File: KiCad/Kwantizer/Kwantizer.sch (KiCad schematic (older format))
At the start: 29 parts

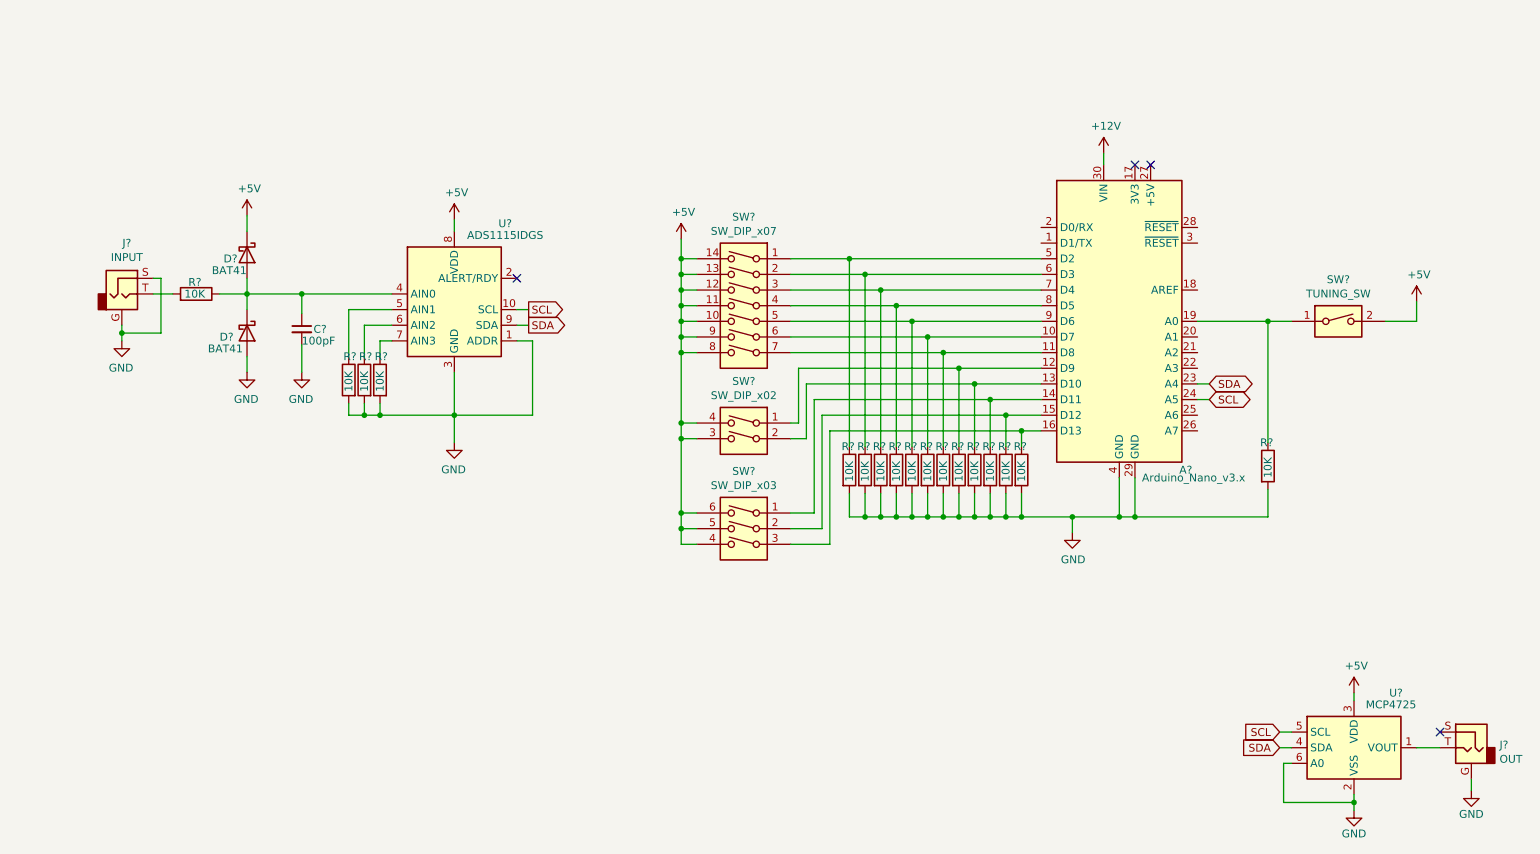
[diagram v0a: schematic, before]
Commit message: Started working on the PCB
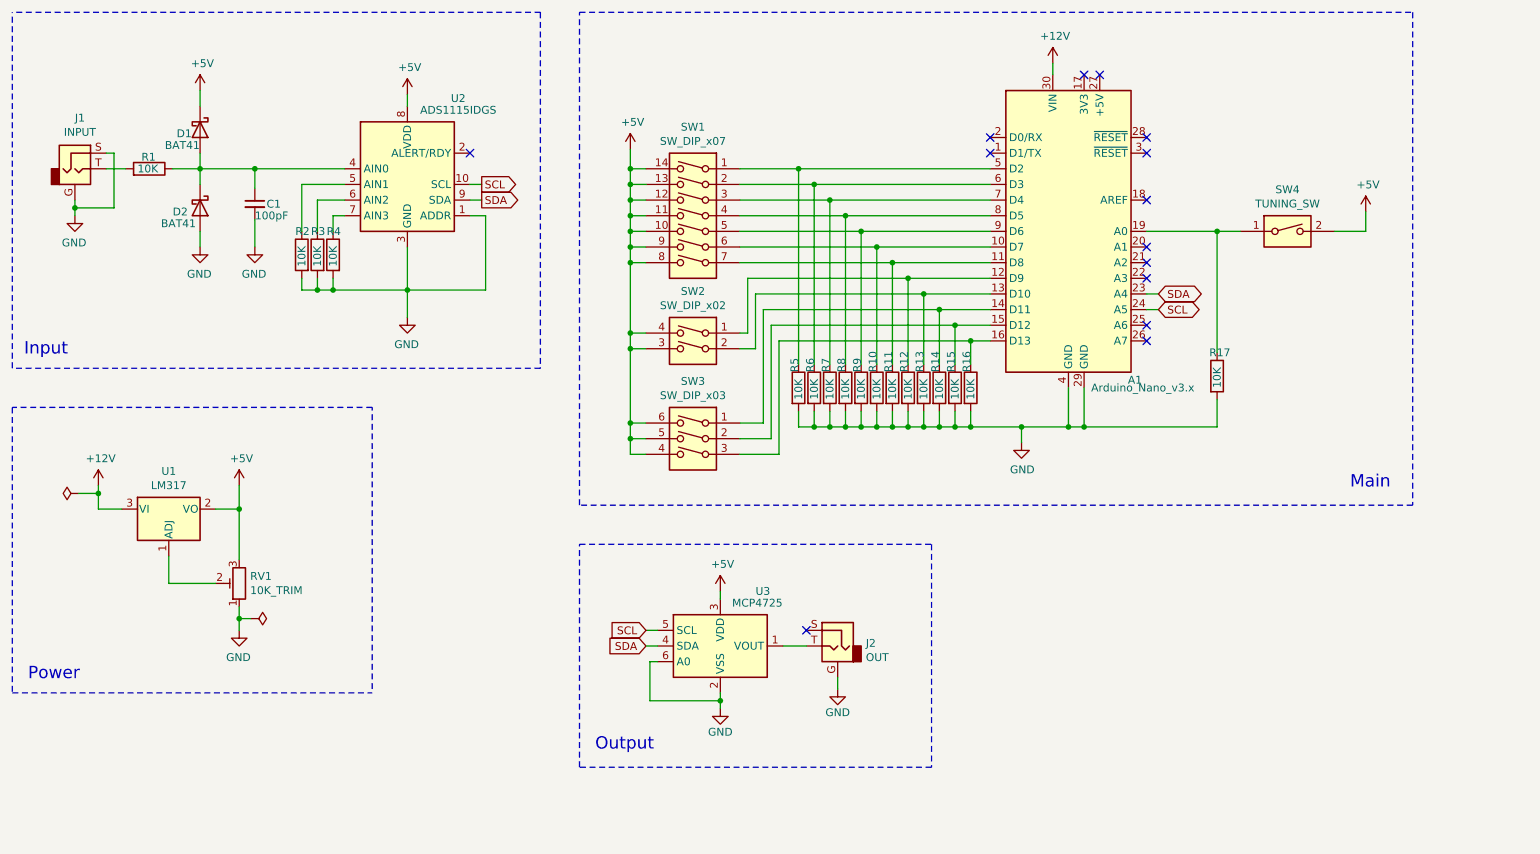
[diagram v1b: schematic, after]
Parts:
- added RV1: 10K_TRIM, Potentiometer_THT:Potentiometer_Bourns_3266Y_Vertical, symbol Device:R_POT_TRIM
- added U1: LM317, Package_TO_SOT_THT:TO-92_Inline, symbol Regulator_Linear:LM317L_TO92
- C1: renamed from C?; footprint (none) -> benjiaomodular:Capacitor_Disc_D3.8mm_W2.6mm_P2.50mm
- J1, J2: renamed from J?; footprint (none) -> benjiaomodular:AudioJack_3.5mm
- R1, R10, R11, R12, R13, R14, R15, R16, R17, R2, R3, R4, R5, R6, R7, R8, R9: renamed from R?; footprint (none) -> benjiaomodular:Resistor_L6.3mm_D2.5mm_P7.62mm_Horizontal
- SW1: renamed from SW?; footprint Package_DIP:SMDIP-14_W7.62mm -> Button_Switch_THT:SW_DIP_SPSTx07_Slide_9.78x19.96mm_W7.62mm_P2.54mm
- SW2: renamed from SW?; footprint (none) -> Button_Switch_THT:SW_DIP_SPSTx02_Slide_9.78x7.26mm_W7.62mm_P2.54mm
- SW3: renamed from SW?; footprint (none) -> Button_Switch_THT:SW_DIP_SPSTx03_Slide_9.78x9.8mm_W7.62mm_P2.54mm
- SW4: renamed from SW?; footprint (none) -> Button_Switch_THT:SW_DIP_SPSTx01_Slide_6.7x4.1mm_W7.62mm_P2.54mm_LowProfile
- gave numbers to parts that had none: 5
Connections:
- net +12V: now also U1.3 (VI)
- net +5V: now also RV1.3, U1.2 (VO)
- net GND: now also RV1.1
- new net: RV1.2, U1.1 (ADJ)
- no-connect marks 4 -> 14
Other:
- note added: "Input"
- note added: "Main"
- note added: "Output"
- note added: "Power"
- moved on the sheet: A1, C1, D1, D2, J1, J2, R1, R10, R11, R12, R13, R14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
